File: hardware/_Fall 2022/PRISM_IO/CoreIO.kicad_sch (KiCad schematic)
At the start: 21 parts, among them J1 Conn_01x07_Female, Q1 Q_NJFET_DGS, Q2 Q_NJFET_DGS, SW1 SW_SPST, SW2 SW_SPST, U1 XT30UPB-M, U2 XT30UPB-M

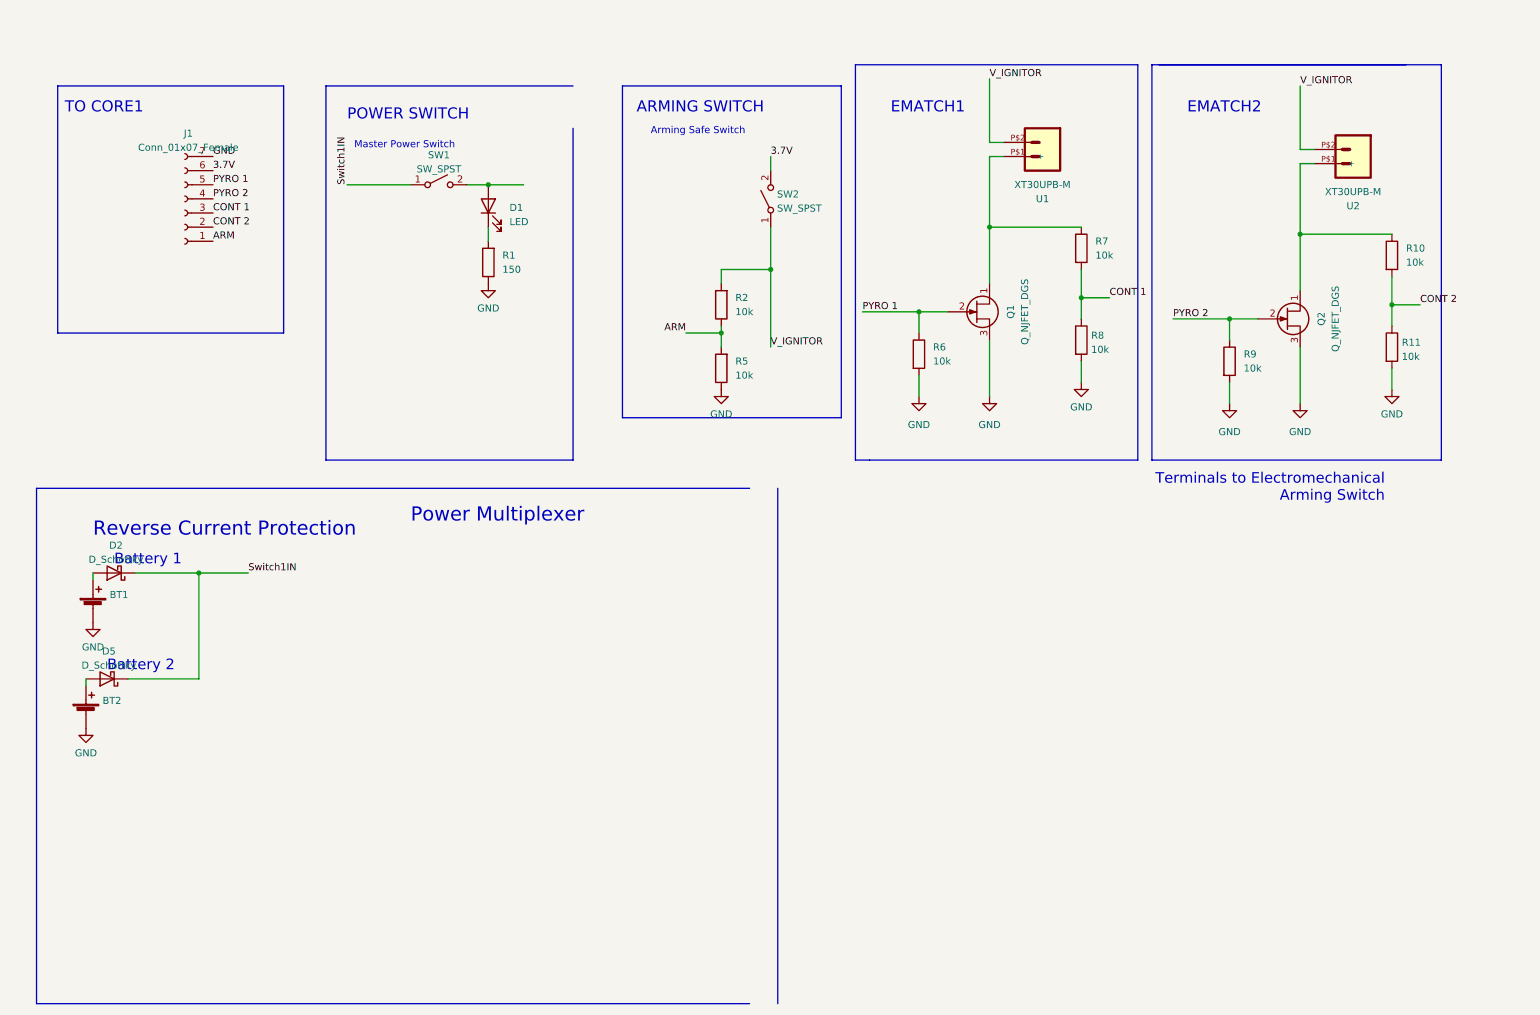
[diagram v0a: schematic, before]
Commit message: work on PRISM io
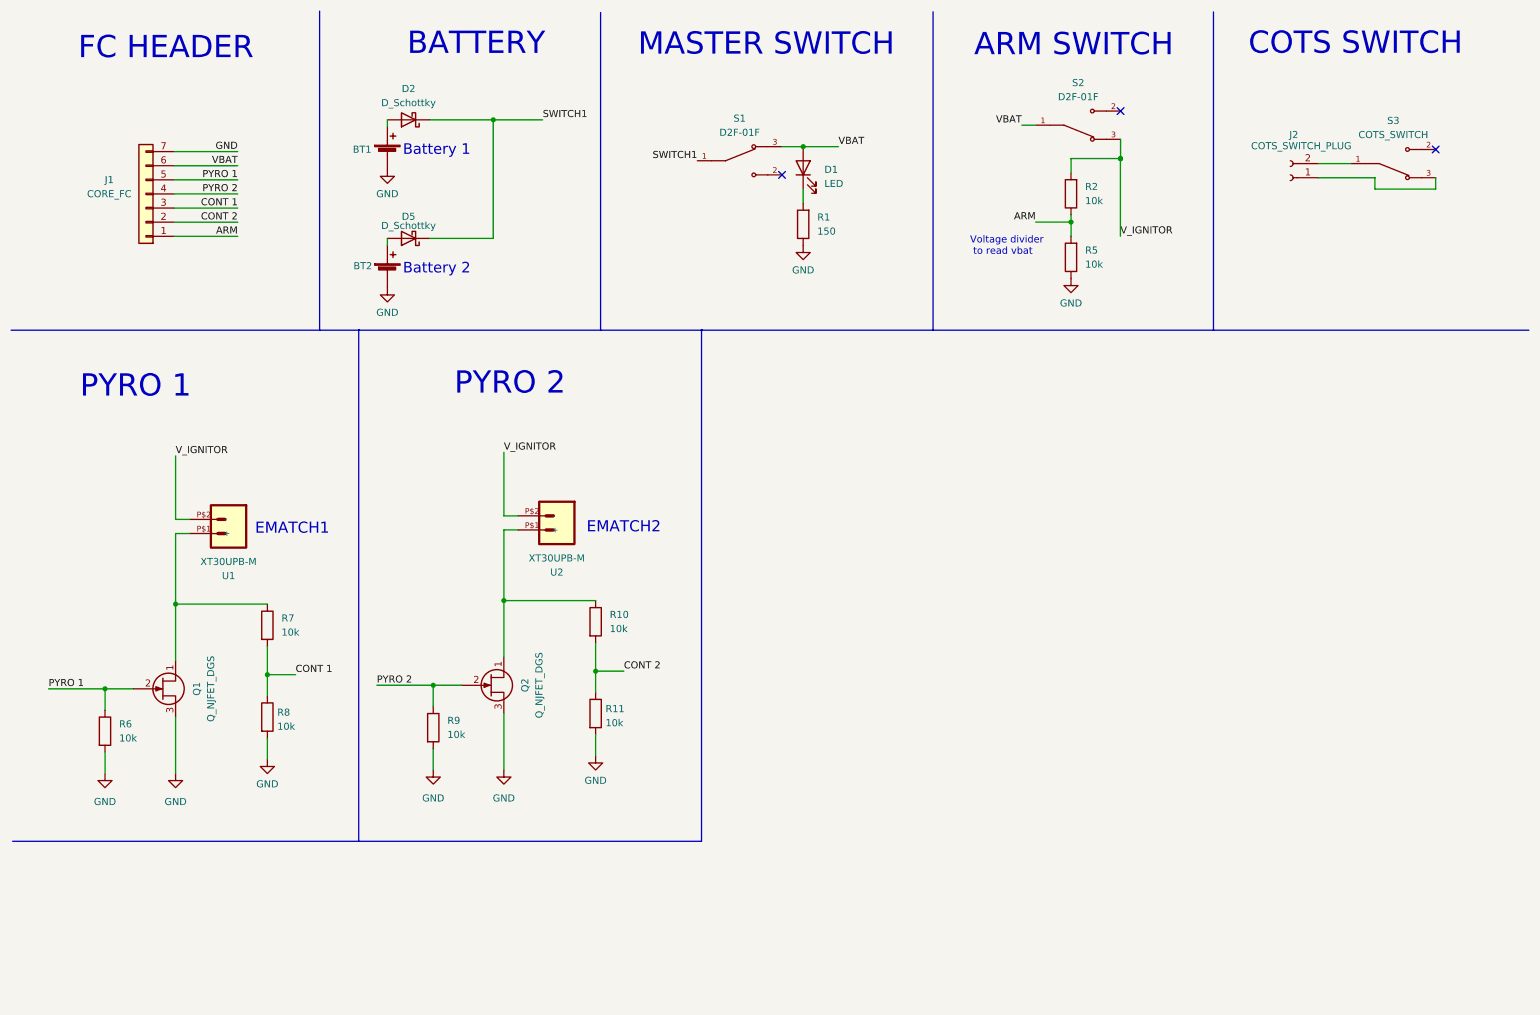
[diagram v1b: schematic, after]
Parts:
- removed J1: Conn_01x07_Female, symbol Connector:Conn_01x07_Female
- removed SW1, SW2: SW_SPST, symbol Switch:SW_SPST
- added J1: CORE_FC, Connector_JST:JST_PH_S7B-PH-K_1x07_P2.00mm_Horizontal, symbol Connector_Generic:Conn_01x07
- added J2: COTS_SWITCH_PLUG, Connector_JST:JST_PH_S2B-PH-K_1x02_P2.00mm_Horizontal, symbol Connector:Conn_01x02_Female
- added S1, S2: D2F-01F, SW_D2F-01F, symbol omron_D2F:D2F-01F
- added S3: COTS_SWITCH, SW_D2F-01F, symbol omron_D2F:D2F-01F
- BT1, BT2: footprint (none) -> JST:JST_SFH_SM02B-SFHRS-TF_02x1.80mm_Angled
- D1: footprint (none) -> LED_SMD:LED_0603_1608Metric
- D2, D5: footprint (none) -> Diode_THT:D_5KPW_P12.70mm_Horizontal
- R1, R10, R11, R2, R5, R6, R7, R8, R9: footprint (none) -> Resistor_SMD:R_0201_0603Metric
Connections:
- net ARM: now also J1.1 (Pin_1)
- net CONT 1: now also J1.3 (Pin_3)
- net CONT 2: now also J1.2 (Pin_2)
- net GND: now also J1.7 (Pin_7)
- net PYRO 1: now also J1.5 (Pin_5)
- net PYRO 2: now also J1.4 (Pin_4)
- net VBAT: now reaches D1.2 (A)
- net VBAT: now also J1.6 (Pin_6), S1.3, S2.1
- net Switch1IN renamed SWITCH1
- net SWITCH1: now also S1.1
- new net: J2.2 (Pin_2), S3.1
- new net: J2.1 (Pin_1), S3.3
- no-connect marks 0 -> 3
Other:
- note added: "ARM SWITCH"
- note added: "BATTERY"
- note added: "COTS SWITCH"
- note added: "FC HEADER"
- note added: "MASTER SWITCH"
- note added: "PYRO 1"
- note added: "PYRO 2"
- note added: "Voltage divider to read vbat"
- note removed: "ARMING SWITCH"
- note removed: "Arming Safe Switch"
- note removed: "Master Power Switch"
- note removed: "POWER SWITCH"
- note removed: "Power Multiplexer"
- note removed: "Reverse Current Protection"
- note removed: "TO CORE1"
- note removed: "Terminals to Electromechanical Arming Switch"
- moved on the sheet: BT1, BT2, D1, D2, D5, Q1, Q2, R1, R10, R11, R2, R5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
